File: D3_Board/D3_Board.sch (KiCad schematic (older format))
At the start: 38 parts, among them J1 POWER_IN, J10 ACS_SENSOR, J11 H-BRIDGE1, J12 H-BRIDGE2, J13 BUZZER_PIN, J14 MOTOR1_POWER, J15 MOTOR1_OUT, J16 MOTOR2_POW, J17 MOTOR2_OUT, J2 POWER_IN, J3 RASPBERRY_POWER_IN, J4 Raspberry_connection, J5 CURRENT_POWER_IN, J6 LED_Matrix, J7 USB_TTL, J8 MOTOR1, J9 MOTOR2, M1 Motor_Servo, M2 Motor_Servo, Q1 BC546, Q2 BC546, Q3 BC546, Q4 BC546, U1 ChinaBluePill-bluepill-D3_Boa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, U2 LM2596_module, U3 GPS_NEO6M_module, U4 MPU6050_module

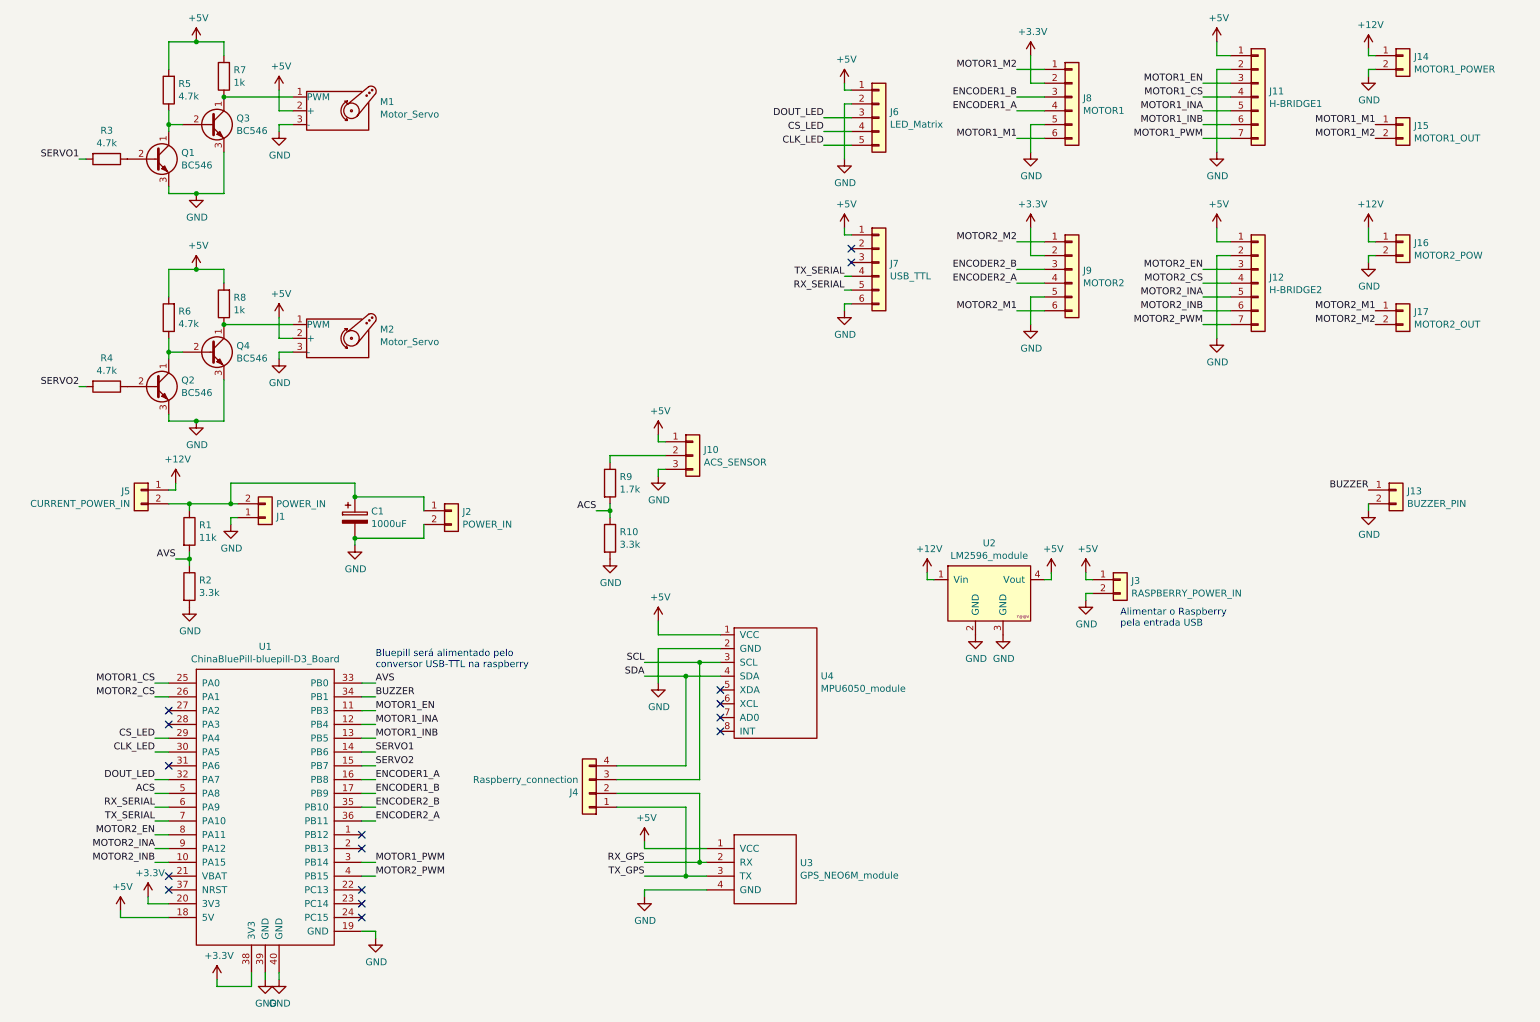
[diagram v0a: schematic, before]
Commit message: Update main board Schematics
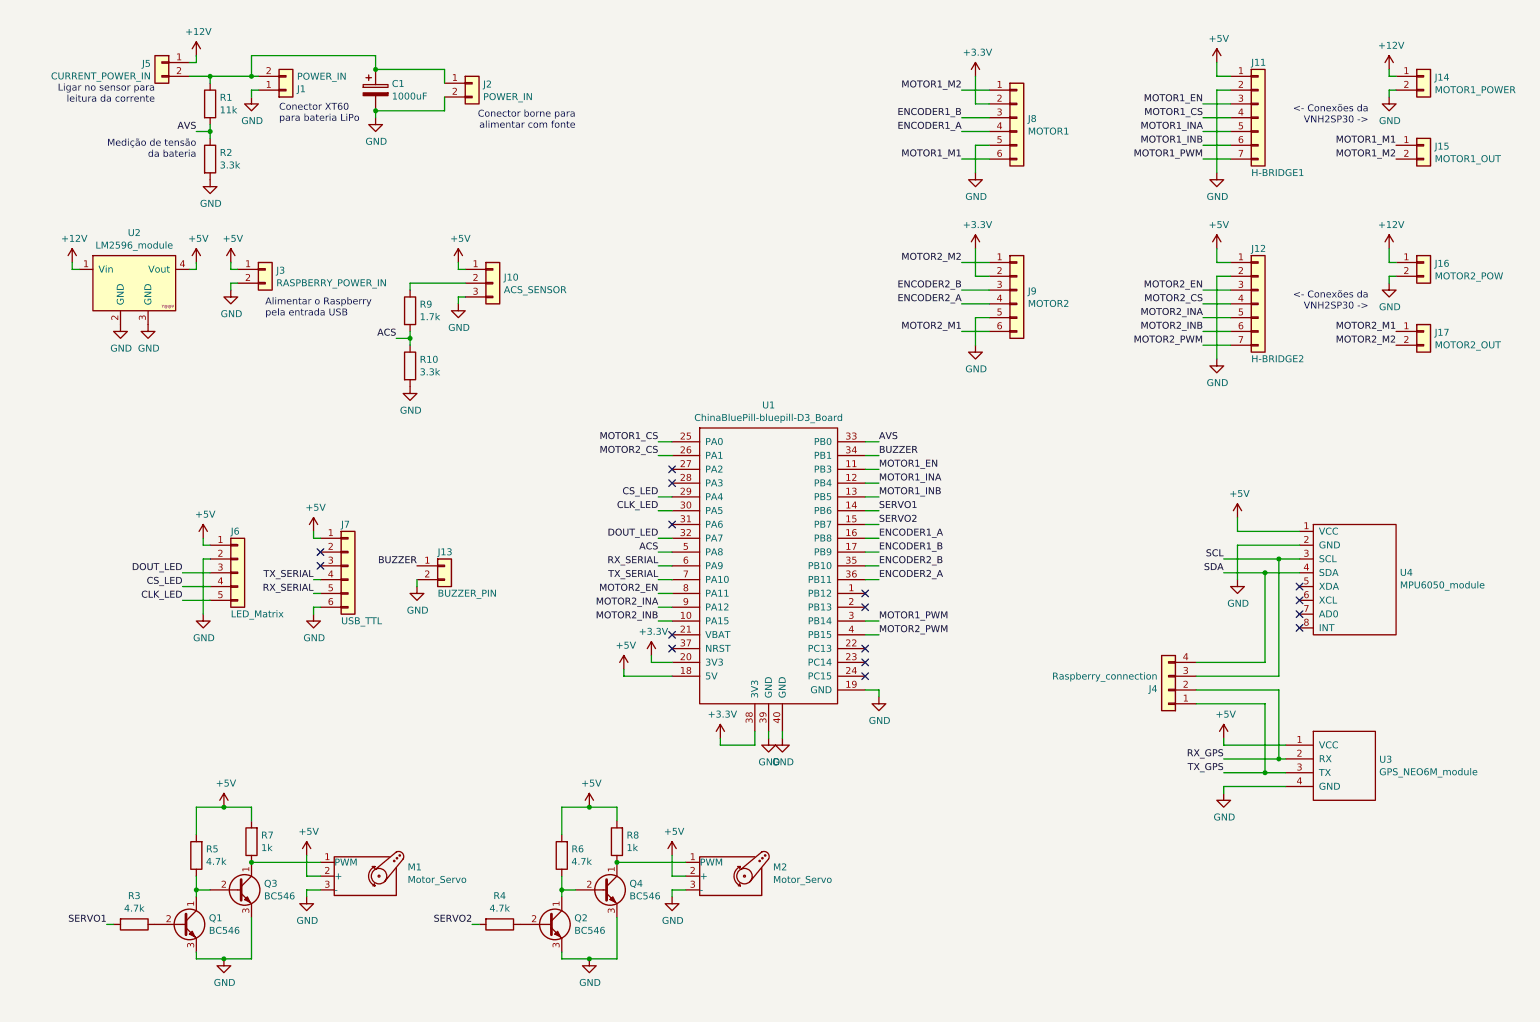
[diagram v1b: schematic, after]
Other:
- note added: "<- Conexões da \nVNH2SP30 ->"
- note added: "Conector XT60 \npara bateria LiPo\n \n\n"
- note added: "Conector borne para\nalimentar com fonte\n \n\n"
- note added: "Ligar no sensor para\nleitura da corrente"
- note added: "Medição de tensão\nda bateria\n"
- note removed: "Bluepill será alimentado pelo\nconversor USB-TTL na raspberry\n"
- moved on the sheet: C1, J1, J10, J11, J12, J13, J14, J15, J16, J17, J2, J3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
